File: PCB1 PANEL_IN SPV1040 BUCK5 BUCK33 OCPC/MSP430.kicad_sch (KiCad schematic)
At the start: 15 parts, among them U20 MSP430F5529IPN, Y1 32K, Y2 CSTCR4M00G53-R0

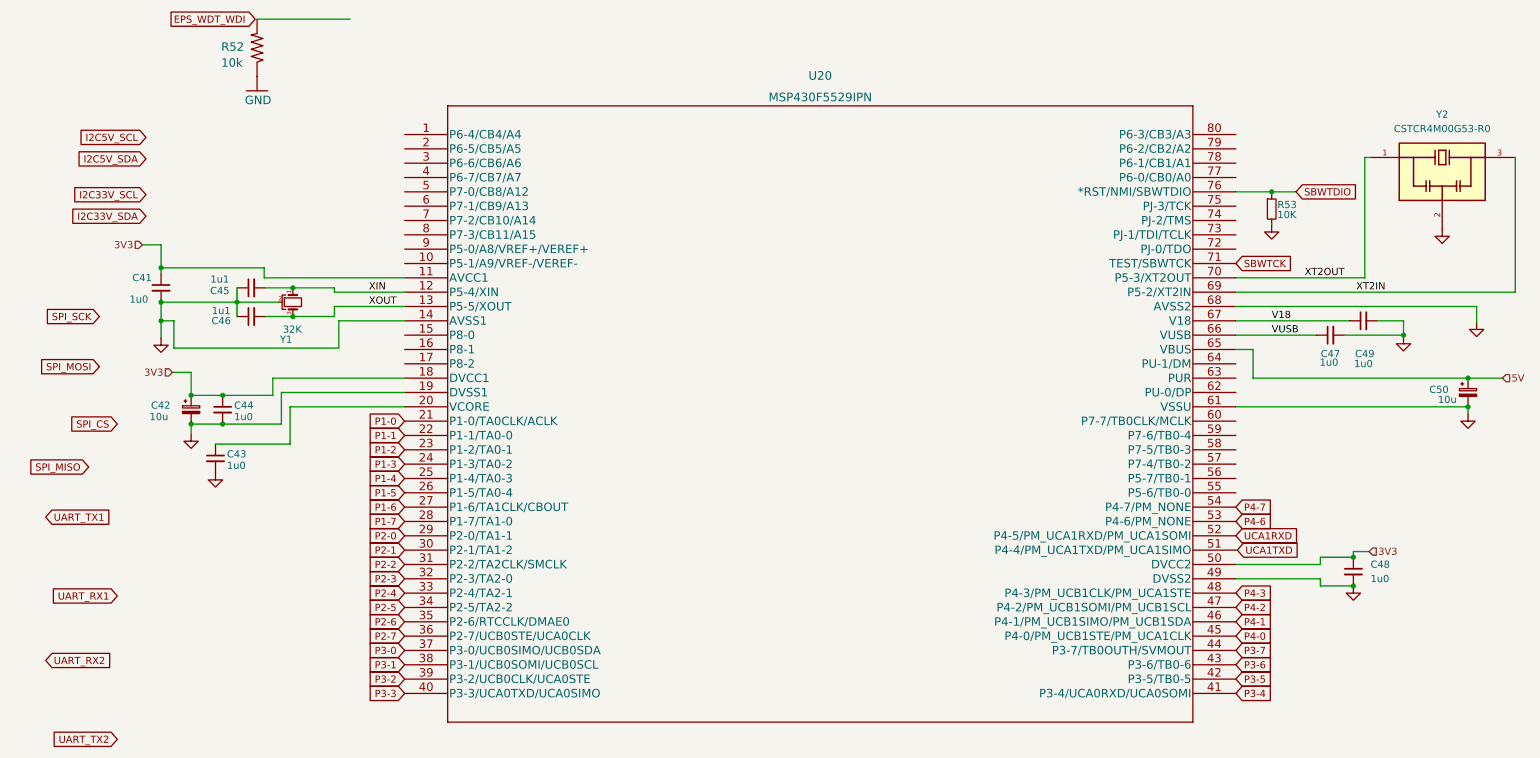
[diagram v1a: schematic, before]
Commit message: Change in MSP sch
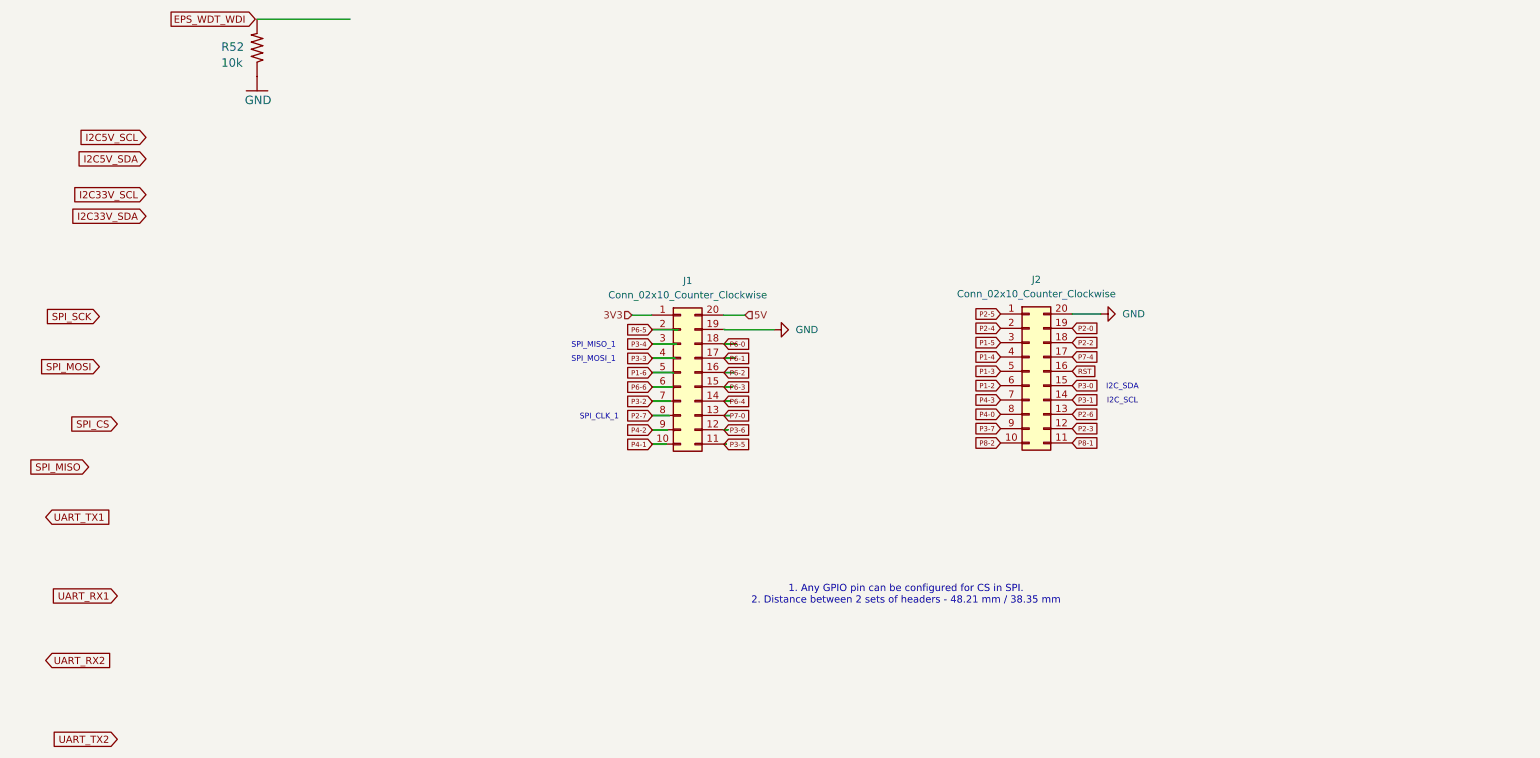
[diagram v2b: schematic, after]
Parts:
- removed C41, C43, C44, C48: 1u0, Capacitor_SMD:C_0603_1608Metric, symbol Device:C_Small
- removed C42: 10u, Capacitor_SMD:CP_Elec_3x5.3, symbol Device:C_Polarized_Small
- removed C45, C46: 1u1, Capacitor_SMD:C_0603_1608Metric, symbol Device:C_Small
- removed C47, C49: 1u0, Capacitor_SMD:C_0402_1005Metric_Pad0.74x0.62mm_HandSolder, symbol Device:C_Small
- removed C50: 10u, Capacitor_SMD:CP_Elec_4x3.9, symbol Device:C_Polarized_Small
- removed R53: 10K, Resistor_SMD:R_0603_1608Metric, symbol Device:R_Small
- removed U20: MSP430F5529IPN, footprintMSP:MSP430F5529IPN, symbol 2023-03-28_15-31-46:MSP430F5529IPN
- removed Y1: 32K, Crystal:Crystal_AT310_D3.0mm_L10.0mm_Horizontal_1EP_style1, symbol Device:Crystal_GND2_Small
- removed Y2: CSTCR4M00G53-R0, CSTCR4M00G53-R0:OSC_CSTCR4M00G53-R0, symbol CSTCR4M00G53-R0:CSTCR4M00G53-R0
- added J1, J2: Conn_02x10_Counter_Clockwise, symbol Connector_Generic:Conn_02x10_Counter_Clockwise
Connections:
- net 3V3: now also J1.1 (Pin_1)
- net 5V: now also J1.20 (Pin_20)
- net GND: now also J1.19 (Pin_19), J2.20 (Pin_20)
- net P1-2: now also J2.6 (Pin_6)
- net P1-3: now also J2.5 (Pin_5)
- net P1-4: now also J2.4 (Pin_4)
- net P1-5: now also J2.3 (Pin_3)
- net P1-6: now also J1.5 (Pin_5)
- net P2-0: now also J2.19 (Pin_19)
- net P2-2: now also J2.18 (Pin_18)
- net P2-3: now also J2.12 (Pin_12)
- net P2-4: now also J2.2 (Pin_2)
- net P2-5: now also J2.1 (Pin_1)
- net P2-6: now also J2.13 (Pin_13)
- net P2-7: now also J1.8 (Pin_8)
- net P3-0: now also J2.15 (Pin_15)
- net P3-1: now also J2.14 (Pin_14)
- net P3-2: now also J1.7 (Pin_7)
- net P3-3: now also J1.4 (Pin_4)
- net P3-4: now also J1.3 (Pin_3)
- net P3-5: now also J1.11 (Pin_11)
- net P3-6: now also J1.12 (Pin_12)
- net P3-7: now also J2.9 (Pin_9)
- net P4-0: now also J2.8 (Pin_8)
- net P4-1: now also J1.10 (Pin_10)
- net P4-2: now also J1.9 (Pin_9)
- net P4-3: now also J2.7 (Pin_7)
- new net P6-0: J1.18 (Pin_18)
- new net P6-1: J1.17 (Pin_17)
- new net P6-2: J1.16 (Pin_16)
- new net P6-3: J1.15 (Pin_15)
- new net P6-4: J1.14 (Pin_14)
- new net P6-5: J1.2 (Pin_2)
- new net P6-6: J1.6 (Pin_6)
- new net P7-0: J1.13 (Pin_13)
- new net P7-4: J2.17 (Pin_17)
- new net P8-1: J2.11 (Pin_11)
- new net P8-2: J2.10 (Pin_10)
- new net RST: J2.16 (Pin_16)
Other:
- note added: "1. Any GPIO pin can be configured for CS in SPI. 2. Distance between 2 sets of headers - 48.21 mm / 38.35 mm"
- note added: "I2C_SCL"
- note added: "I2C_SDA"
- note added: "SPI_CLK_1"
- note added: "SPI_MISO_1"
- note added: "SPI_MOSI_1"
